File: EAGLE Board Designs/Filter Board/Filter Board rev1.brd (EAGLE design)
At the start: 50.8 x 152.4 mm, 124 parts, among them J4 CONNECTOR-40__, J5 CONNECTOR-40__, U10 MAX7400, U11 MAX7400, U19 MAX7400, U20 MAX7400, U21 MAX7400, U22 MAX7400, U23 MAX7400, U24 MAX7400, U6 MAX7400, U7 MAX7400, U8 MAX7400, U9 MAX7400

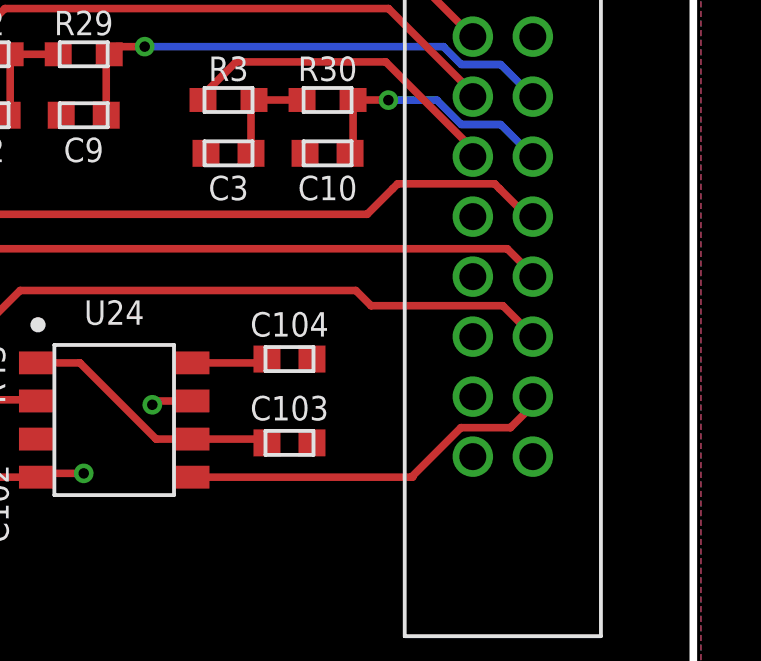
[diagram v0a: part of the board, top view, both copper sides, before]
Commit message: embarassing
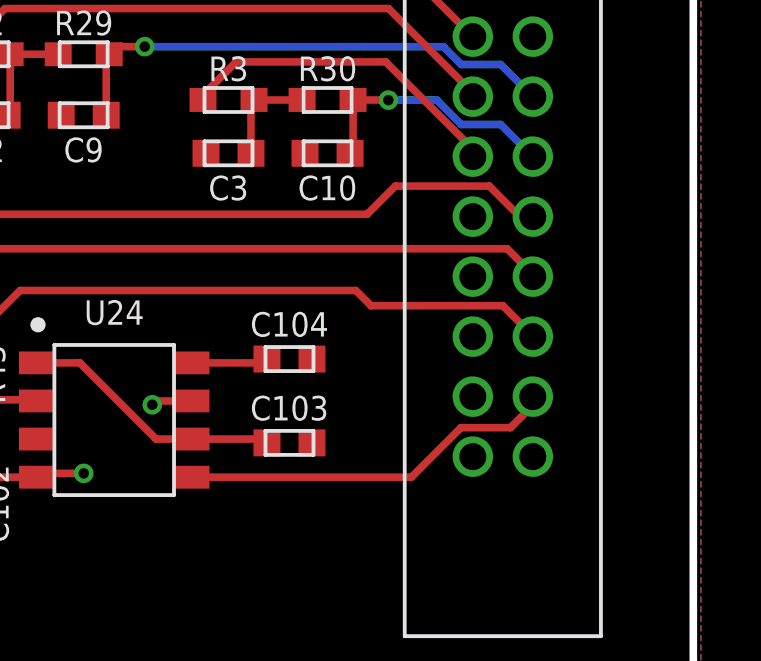
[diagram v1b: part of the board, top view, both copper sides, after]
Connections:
- net GND: now also R42.2
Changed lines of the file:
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@@
 <contactref element="R18" pad="2"/>
 <contactref element="R44" pad="2"/>
+<contactref element="R42" pad="2"/>
 </signal>
 <signal name="LOAD_FL_EXT">
@@
 <contactref element="R41" pad="1"/>
 <wire x1="7.62" y1="35.394" x2="7.62" y2="36.156" width="0.254" layer="1"/>
-<wire x1="45.27180625" y1="38.53" x2="45.45" y2="38.53" width="0.254" layer="1"/>
-<wire x1="45.27180625" y1="38.53" x2="44.34280625" y2="39.459" width="0.254" layer="1"/>
+<wire x1="45.01780625" y1="38.53" x2="45.45" y2="38.53" width="0.254" layer="1"/>
+<wire x1="45.01780625" y1="38.53" x2="44.00000625" y2="39.5478" width="0.254" layer="1"/>
 <wire x1="7.62" y1="36.156" x2="10.072" y2="38.608" width="0.254" layer="1"/>
 <wire x1="10.072" y1="38.608" x2="39.92819375" y2="38.608" width="0.254" layer="1"/>
-<wire x1="40.77919375" y1="39.459" x2="39.92819375" y2="38.608" width="0.254" layer="1"/>
-<wire x1="44.34280625" y1="39.459" x2="44.17780625" y2="39.624" width="0.254" layer="1"/>
-<wire x1="40.94419375" y1="39.624" x2="40.77919375" y2="39.459" width="0.254" layer="1"/>
-<wire x1="44.17780625" y1="39.624" x2="40.94419375" y2="39.624" width="0.254" layer="1"/>
+<wire x1="40.86799375" y1="39.5478" x2="39.92819375" y2="38.608" width="0.254" layer="1"/>
+<wire x1="44.00000625" y1="39.5478" x2="40.86799375" y2="39.5478" width="0.254" layer="1"/>
 </signal>
 <signal name="REFERENCE_EXT">
@@
 <contactref element="U24" pad="5"/>
 <wire x1="34.0995" y1="29.845" x2="41.402" y2="29.845" width="0.254" layer="1"/>
-<wire x1="41.402" y1="29.845" x2="41.45119375" y2="29.845" width="0.254" layer="1"/>
 <wire x1="41.402" y1="29.845" x2="43.053" y2="31.496" width="0.254" layer="1"/>
 <wire x1="43.053" y1="31.496" x2="44.704" y2="31.496" width="0.254" layer="1"/>
